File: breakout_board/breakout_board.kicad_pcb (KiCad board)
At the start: 4 copper layers, 30.2 x 37.9 mm, 54 parts, among them J1 Conn_01x14, J2 Conn_01x14, J3 CONN_01X03, J4 CONN_02x04, J5 Conn_01x04, U1 TB6612FNG, U2 LP5907SNX-3.3/NOPB, U3 LSF0204RUTR, U4 ADP3330, U5 TLV70718PDQNR

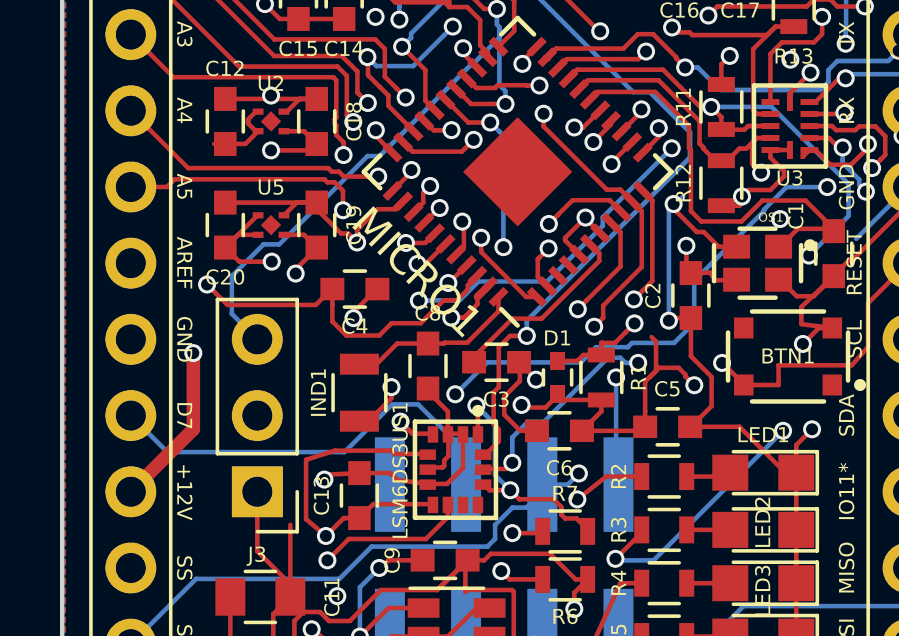
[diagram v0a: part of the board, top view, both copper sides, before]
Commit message: did DRC
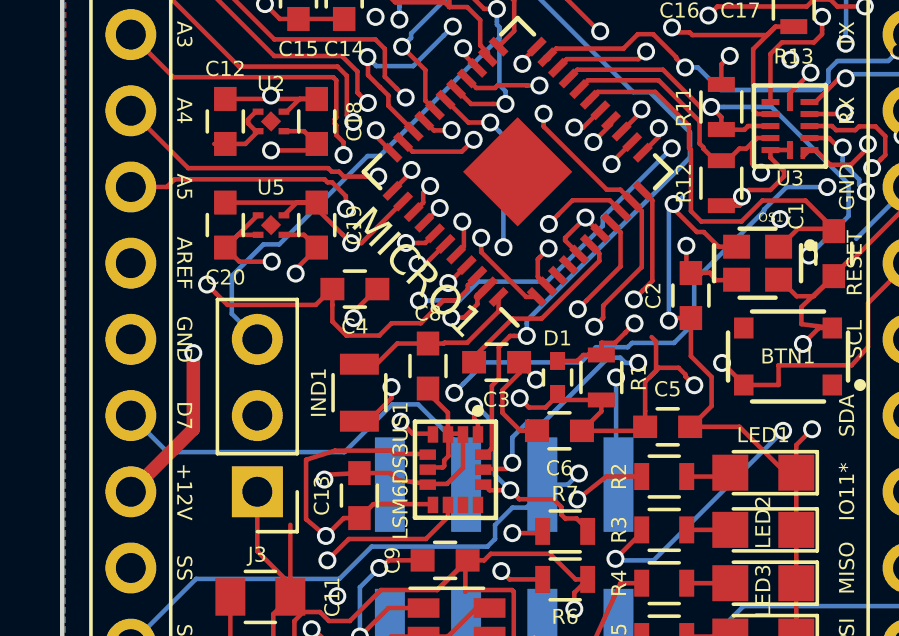
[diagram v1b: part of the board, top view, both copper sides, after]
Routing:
- net /TXLED: track 27.0 -> 26.3 mm
